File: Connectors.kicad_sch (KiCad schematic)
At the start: 4 parts, among them J1 Conn_01x04_Pin, J2 Conn_01x04_Pin, J3 Conn_01x09_Pin, J4 Conn_02x03_Odd_Even

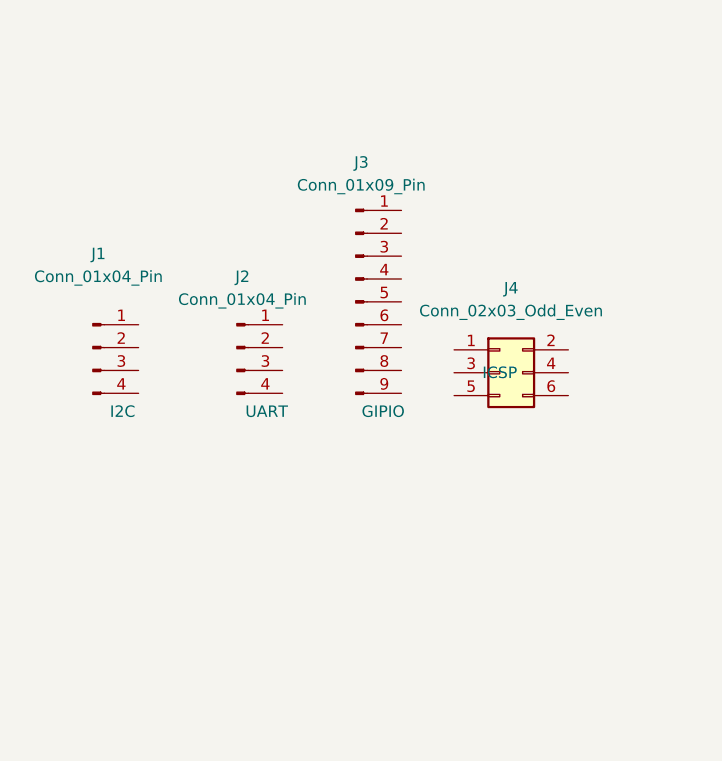
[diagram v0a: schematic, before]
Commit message: schematic done
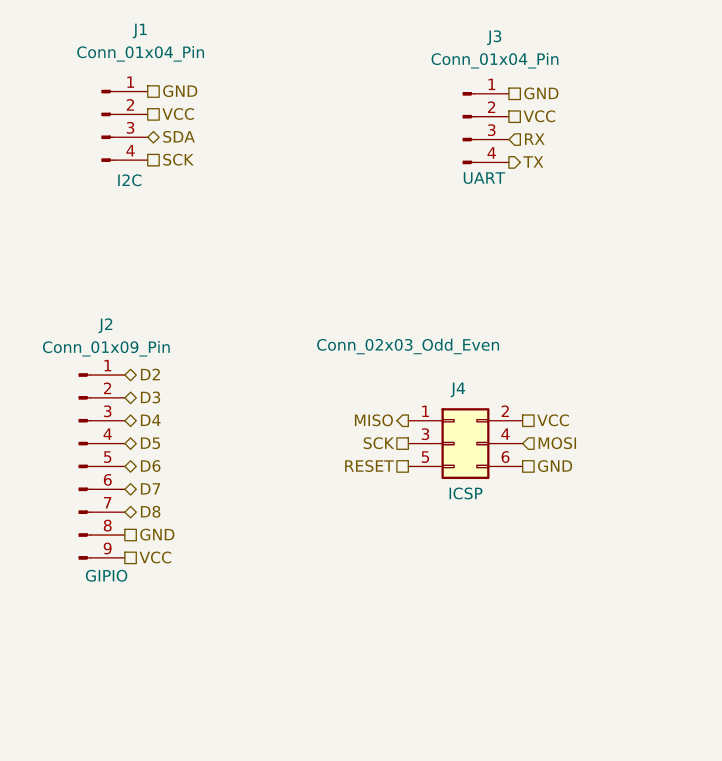
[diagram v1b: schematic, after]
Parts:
- renumbered J3 to J2, J2 to J3
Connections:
- net D2: now reaches J2.1 (Pin_1)
- net D3: now reaches J2.2 (Pin_2)
- net D4: now reaches J2.3 (Pin_3)
- net D5: now reaches J2.4 (Pin_4)
- net D6: now reaches J2.5 (Pin_5)
- net D7: now reaches J2.6 (Pin_6)
- net D8: now reaches J2.7 (Pin_7)
- net GND: now reaches J2.8 (Pin_8)
- net GND: now also J1.1 (Pin_1), J3.1 (Pin_1), J4.6 (Pin_6)
- net VCC: now reaches J2.9 (Pin_9)
- net VCC: now also J1.2 (Pin_2), J3.2 (Pin_2), J4.2 (Pin_2)
- net SDA: now reaches J1.3 (Pin_3)
- net SCK: now reaches J1.4 (Pin_4)
- net SCK: now also J4.3 (Pin_3)
- net MISO: now reaches J4.1 (Pin_1)
- net MOSI: now reaches J4.4 (Pin_4)
- net RESET: now reaches J4.5 (Pin_5)
- net RX: now reaches J3.3 (Pin_3)
- net TX: now reaches J3.4 (Pin_4)
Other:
- moved on the sheet: J1, J2, J3, J4

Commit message: copied the schematic
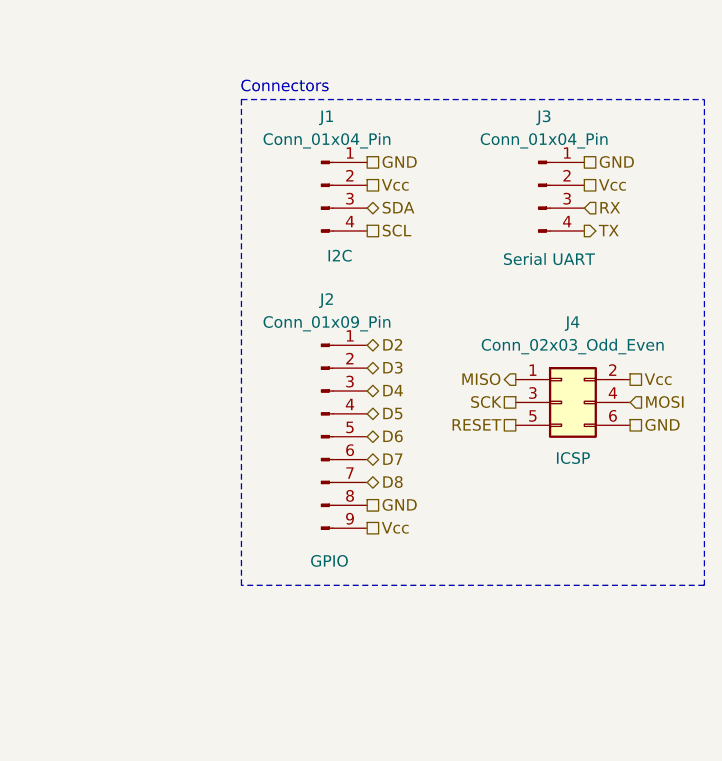
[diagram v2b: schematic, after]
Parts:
- J2: Purpose GIPIO -> GPIO
- J3: Purpose UART -> Serial UART
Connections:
- net SCK: no longer J1.4 (Pin_4)
- net VCC renamed Vcc
- new net SCL: J1.4 (Pin_4)
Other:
- note added: "Connectors"

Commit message: şematik tamamalandı
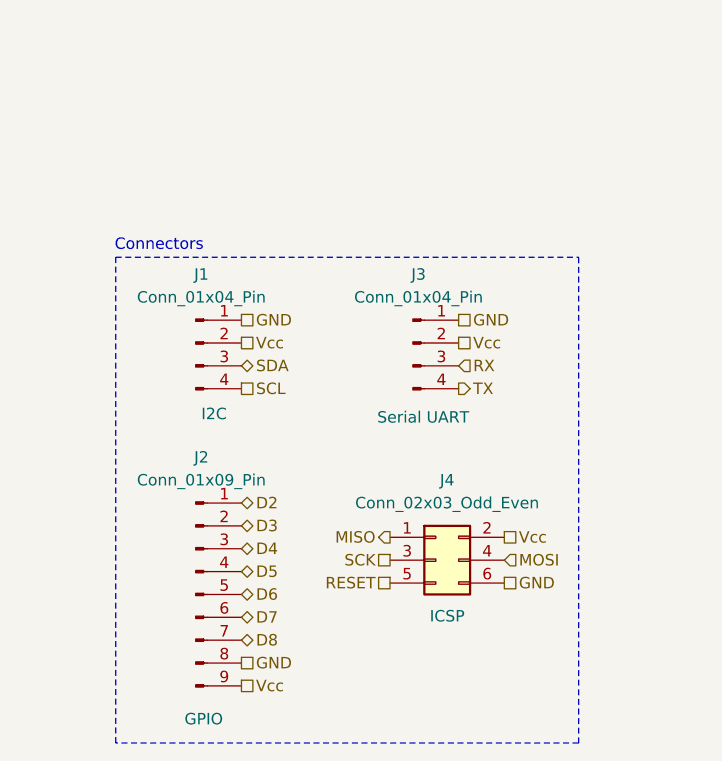
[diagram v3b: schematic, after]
